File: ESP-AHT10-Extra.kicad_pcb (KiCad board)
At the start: 2 copper layers, 38.2 x 20.8 mm, 29 parts, among them J1 USB, SW1 RESET, SW2 PROG, U1 CH330N, U2 HT7233, U3 ESP-12, U4 AHT10, U5 USBLC6-2SC6

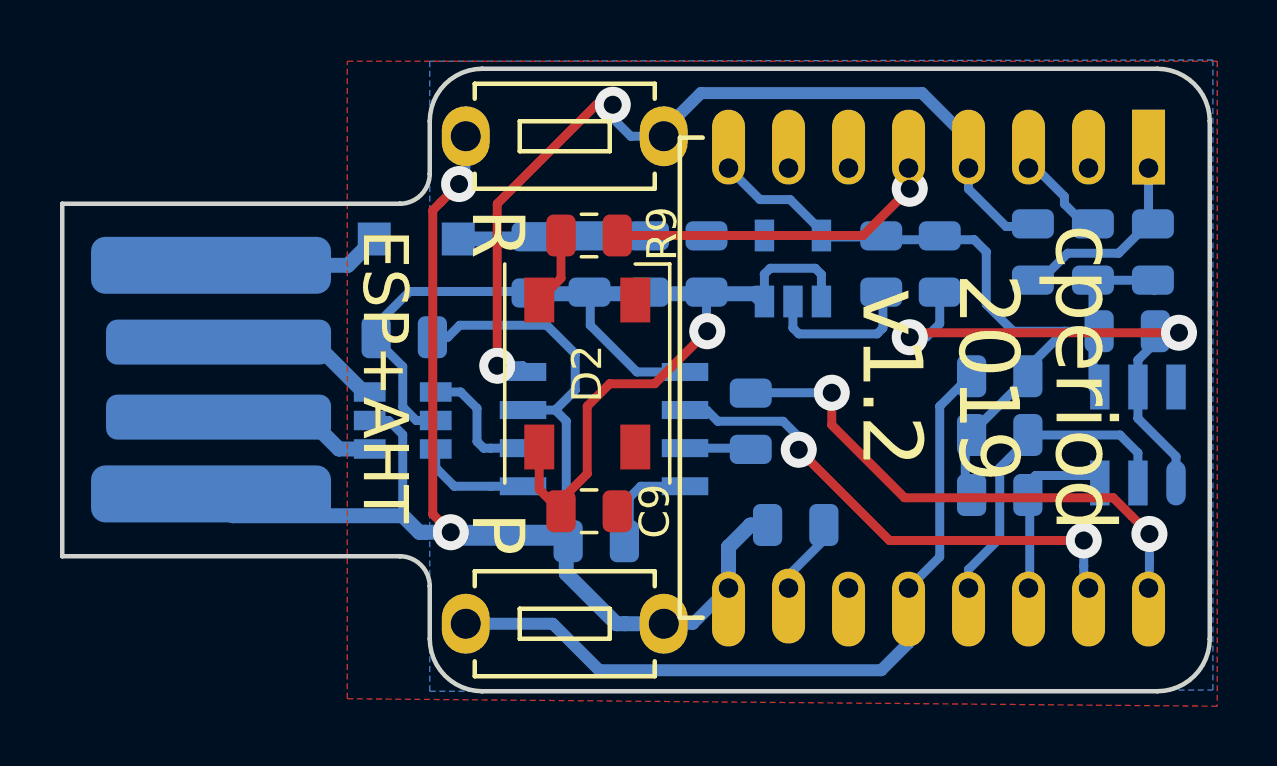
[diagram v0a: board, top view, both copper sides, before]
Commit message: more tweaking
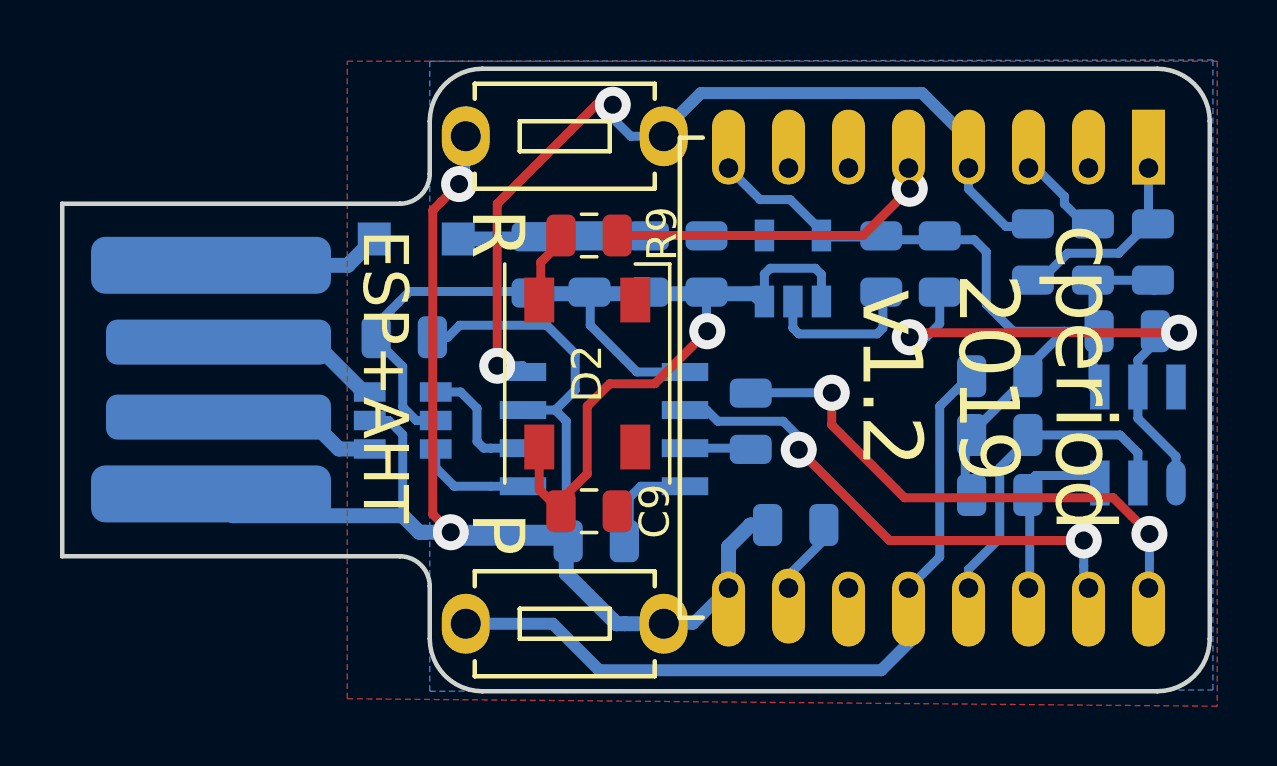
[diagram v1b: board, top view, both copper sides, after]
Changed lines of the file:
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@@
     (thickness 1.6)
     (drawings 19)
-    (tracks 233)
+    (tracks 235)
     (zones 0)
     (modules 29)
@@
   )
   (layers
-    (0 F.Cu signal hide)
-    (31 B.Cu signal)
+    (0 F.Cu signal)
+    (31 B.Cu signal hide)
     (32 B.Adhes user hide)
     (33 F.Adhes user hide)
-    (34 B.Paste user)
-    (35 F.Paste user hide)
-    (36 B.SilkS user)
-    (37 F.SilkS user hide)
-    (38 B.Mask user)
-    (39 F.Mask user hide)
+    (34 B.Paste user hide)
+    (35 F.Paste user)
+    (36 B.SilkS user hide)
+    (37 F.SilkS user)
+    (38 B.Mask user hide)
+    (39 F.Mask user)
     (40 Dwgs.User user hide)
     (41 Cmts.User user hide)
@@
     (44 Edge.Cuts user)
     (45 Margin user hide)
-    (46 B.CrtYd user)
-    (47 F.CrtYd user hide)
-    (48 B.Fab user)
-    (49 F.Fab user hide)
+    (46 B.CrtYd user hide)
+    (47 F.CrtYd user)
+    (48 B.Fab user hide)
+    (49 F.Fab user)
   )
   (setup
@@
   (segment (start 162.355703 92.25862) (end 161.45862 92.25862) (width 0.3) (layer B.Cu) (net 20))
   (segment (start 161.45862 92.25862) (end 160.209217 91.009217) (width 0.3) (layer B.Cu) (net 20))
-  (segment (start 146.625 93.985001) (end 145.9 94.710001) (width 0.3) (layer F.Cu) (net 21))
-  (segment (start 146.625 92.55862) (end 146.625 93.985001) (width 0.3) (layer F.Cu) (net 21))
+  (segment (start 145.95 94.660001) (end 145.9 94.710001) (width 0.3) (layer F.Cu) (net 21))
+  (segment (start 145.95 93.45) (end 145.95 94.660001) (width 0.3) (layer F.Cu) (net 21))
+  (segment (start 146.625 92.55862) (end 146.625 92.775) (width 0.3) (layer F.Cu) (net 21))
+  (segment (start 146.625 92.775) (end 145.95 93.45) (width 0.3) (layer F.Cu) (net 21))
   (segment (start 158.209217 90.312374) (end 158.187626 90.312374) (width 0.3) (layer F.Cu) (net 22))
   (via (at 158.25 91) (size 1.2) (drill 0.6) (layers F.Cu B.Cu) (net 22))
